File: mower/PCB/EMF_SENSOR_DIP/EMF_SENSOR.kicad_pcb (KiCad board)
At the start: 2 copper layers, 74.4 x 33 mm, 24 parts, among them J1 Conn_01x03_Pin, U1 LM358, U2 LM393

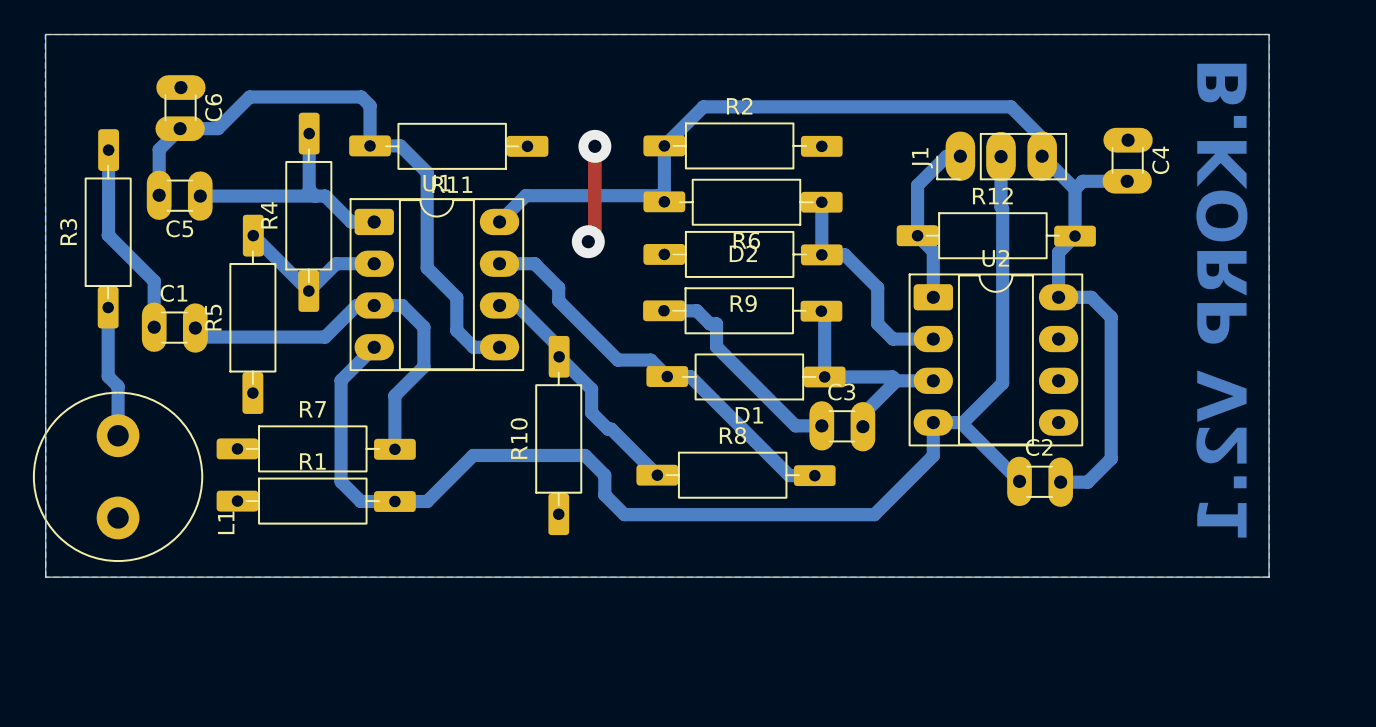
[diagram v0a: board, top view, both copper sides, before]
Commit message: Consolidate complete mower design (all branches) + zana repo structure
Mower fragments from every botkorp branch (mowbot3/4, TRANSMITTER_SMD,
IMRANS_LIBRARY) unioned into mower/. Adds legacy/opengro, README, .gitignore.
Sits on top of the preserved 13-commit mower history.

Co-Authored-By: Claude Opus 4.8 <noreply@anthropic.com>
Claude-Session: https://claude.ai/code/session_017QXBEryTihUadNUZqQzfmo
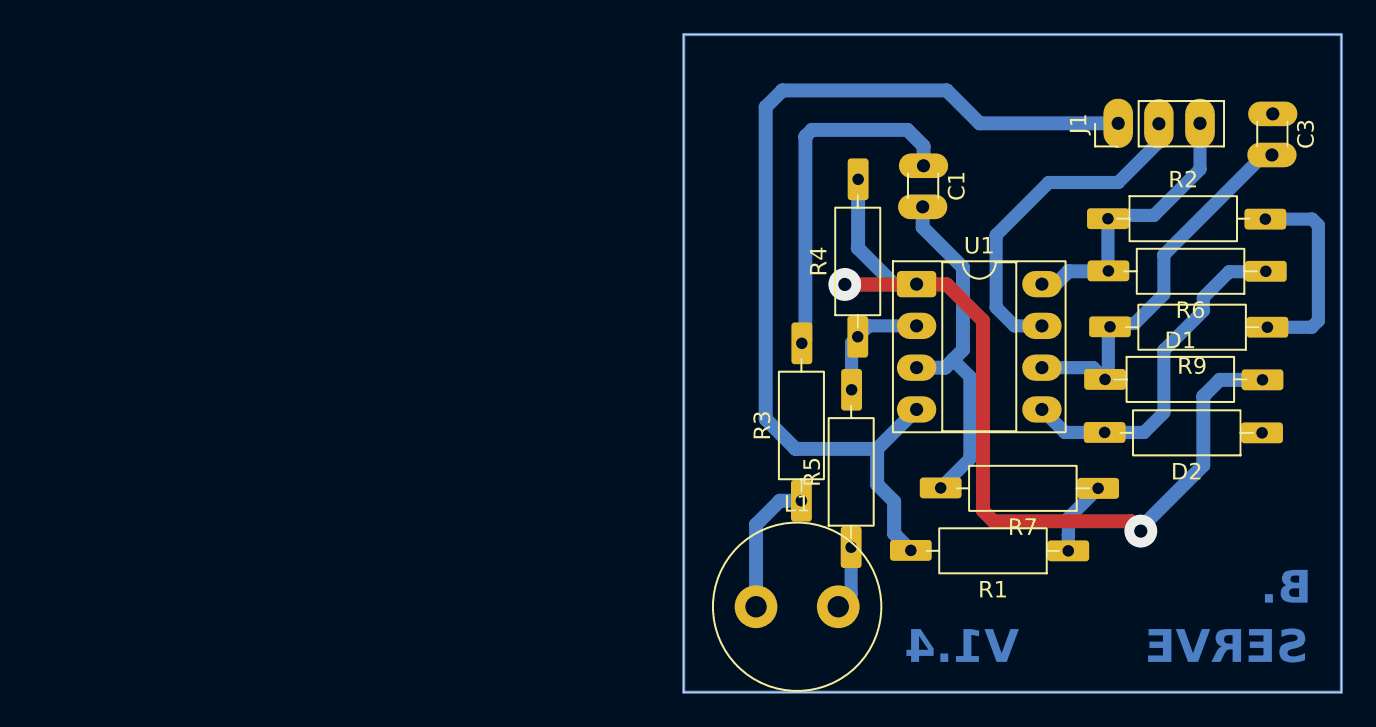
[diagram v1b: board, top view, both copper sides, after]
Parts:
- removed C2, C4: 10uF, IMRANS_LIBRARY:C_Disc_D3.0mm_W1.6mm_P2.50mm
- removed C5: 1nF, IMRANS_LIBRARY:C_Disc_D3.0mm_W1.6mm_P2.50mm
- removed C6: 0.01uF, IMRANS_LIBRARY:C_Disc_D3.0mm_W1.6mm_P2.50mm
- removed R10, R11: 10K, IMRANS_LIBRARY:R_Axial_DIN0207_L6.3mm_D2.5mm_P10.16mm_Horizontal_2
- removed R12: 100K, IMRANS_LIBRARY:R_Axial_DIN0207_L6.3mm_D2.5mm_P10.16mm_Horizontal_2
- removed R8: 1M, IMRANS_LIBRARY:R_Axial_DIN0207_L6.3mm_D2.5mm_P10.16mm_Horizontal_2
- removed U2: LM393, Package_DIP:DIP-8_W7.62mm_Socket_LongPads
- D2: value 1N5819 -> D
- R7: value 10K -> 1K
- moved R7 53.4 mm to (163.7, 65.6), turned to 180 degrees
- moved R1 51.6 mm to (161.9, 69.4), turned to 180 degrees
- moved C1 47.8 mm to (152.6, 46.0), turned to -90 degrees
- moved R3 43.8 mm to (145.2, 66.9)
- moved L1 40.2 mm to (142.4, 72.8), turned to 0 degrees
- moved D2 38.9 mm to (173.7, 62.2), turned to 180 degrees
- moved R9 37.7 mm to (174.0, 55.8), turned to 180 degrees
- moved R5 37.6 mm to (148.2, 69.7)
- moved R4 33.5 mm to (148.6, 56.9)
- moved C3 33.4 mm to (173.8, 42.8), turned to -90 degrees
- moved U1 33.2 mm to (152.2, 53.2)
- moved R2 27.3 mm to (163.3, 49.2)
- moved R6 27.3 mm to (173.9, 52.4)
- moved D1 16.1 mm to (163.1, 59.0), turned to 0 degrees
- moved J1 9.81 mm to (164.4, 43.4)
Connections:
- J1 pad 1: Net-(J1-Pin_1) -> GND
- J1 pad 2: GND -> Net-(J1-Pin_2)
- R4 pad 2: Net-(C5-Pad1) -> Net-(D1-A)
- U1 pad 1: Net-(C5-Pad1) -> Net-(D1-A)
- U1 pad 5: Net-(U1B-+) -> Net-(D2-A)
- U1 pad 6: Net-(U1B--) -> Net-(D1-K)
- U1 pad 7: Net-(D1-A) -> Net-(J1-Pin_2)
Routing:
- net VCC: track 69.3 -> 17.7 mm
- net Net-(U1B-+): track 37.1 -> 0.00 mm
- net Net-(D1-A): track 25.0 -> 57.8 mm, vias 0 -> 2
- net Net-(J1-Pin_2): track 0.00 -> 21.0 mm
- net GND: track 76.4 -> 59.9 mm
- net Net-(U1B--): track 15.9 -> 0.00 mm
- net Net-(C5-Pad1): track 15.2 -> 0.00 mm
- net Net-(J1-Pin_1): track 10.5 -> 0.00 mm
- net Net-(C1-Pad1): track 11.9 -> 21.6 mm
- net Net-(D1-K): track 14.2 -> 23.2 mm
- net Net-(D2-A): track 13.4 -> 20.9 mm
- net Net-(U1A--): track 9.44 -> 7.23 mm
- net Net-(U1A-+): track 23.6 -> 21.9 mm
- net GNDREF: track 19.3 -> 20.9 mm, vias 2 -> 0
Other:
- board size 74.4 x 33 mm -> 40 x 40 mm
- board text added: "B."
- board text added: "SERVE"
- board text added: "V1.4"
- board text removed: "B.KORP V2.1"
